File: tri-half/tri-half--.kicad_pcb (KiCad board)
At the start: 2 copper layers, 43.3 x 50 mm, 11 parts, among them J1 Conn_01x05_Pin, J2 Conn_01x05_Pin, J3 Conn_01x05_Pin

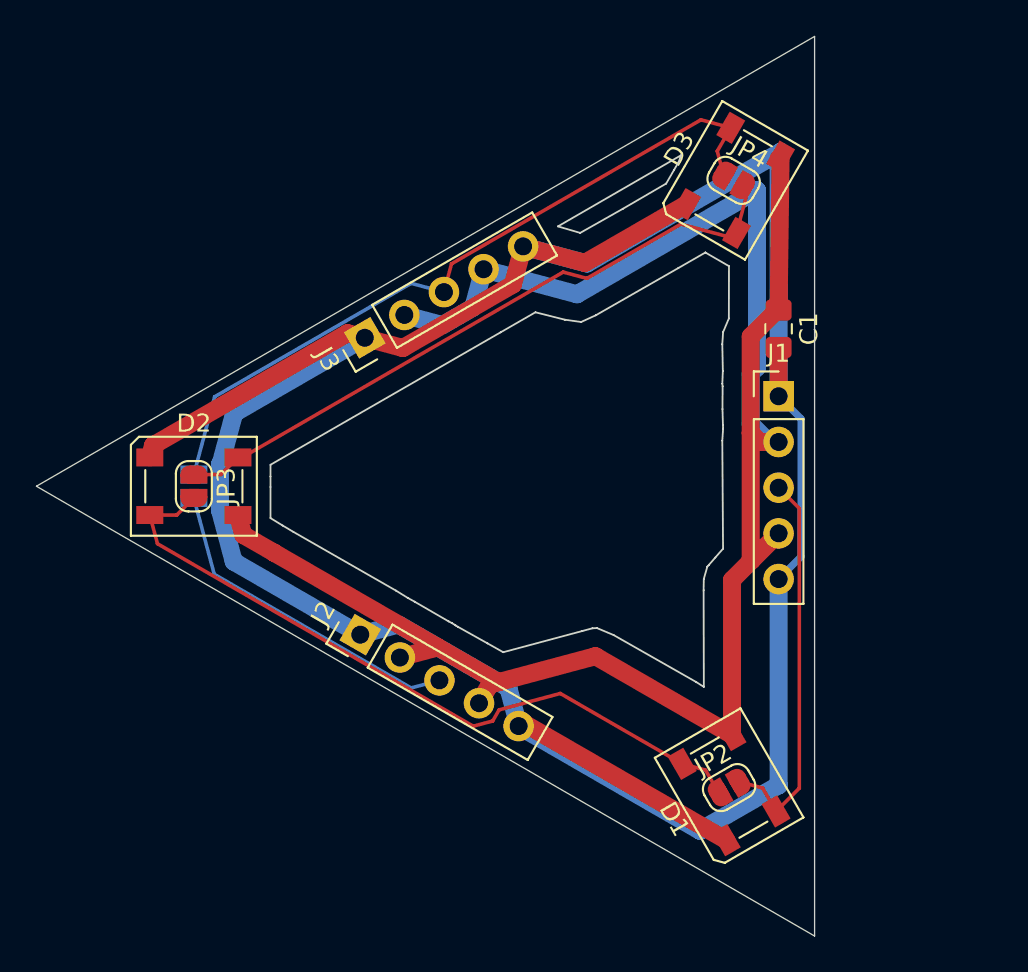
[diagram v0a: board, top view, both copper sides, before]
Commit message: very nice
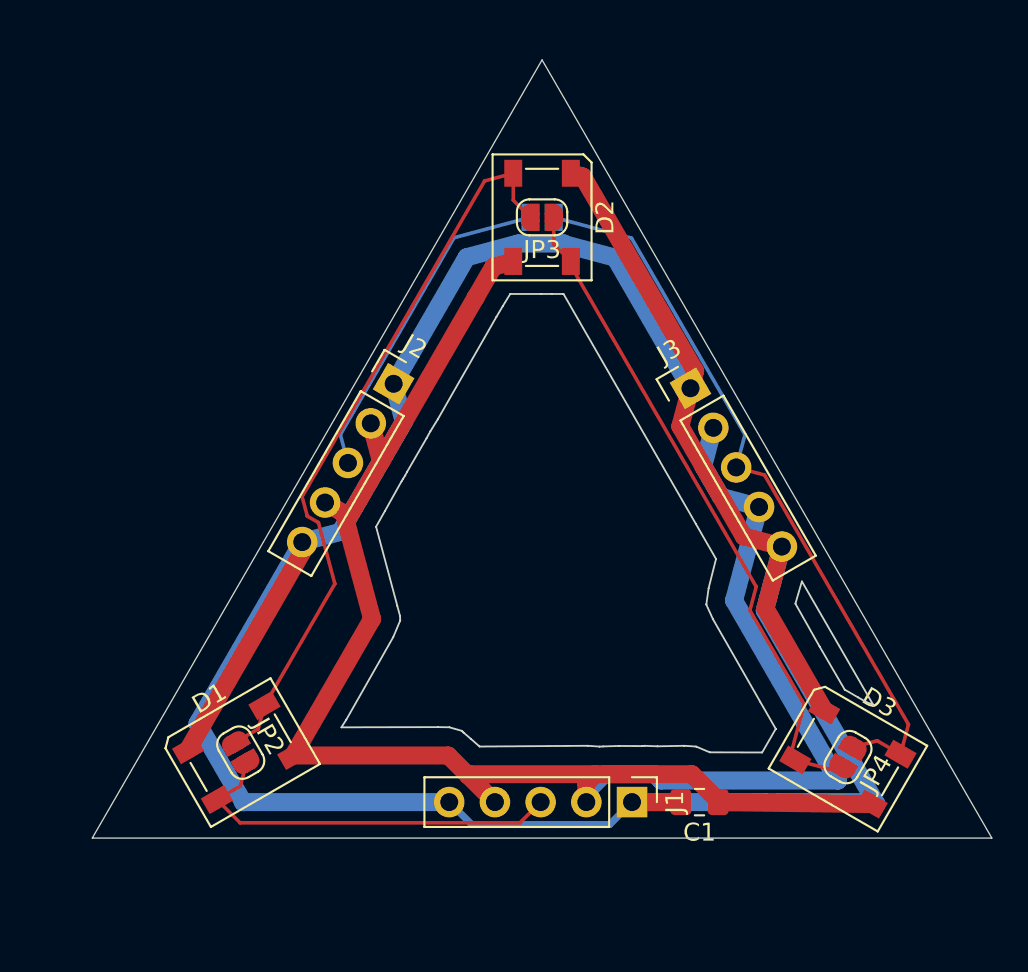
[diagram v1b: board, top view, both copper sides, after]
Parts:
- moved D3 32.7 mm to (116.9, 69.2), turned to -30 degrees
- moved JP4 32.7 mm to (116.9, 69.2), turned to -120 degrees
- moved D1 27.2 mm to (83.1, 68.9), turned to 30 degrees
- moved JP2 27.2 mm to (83.1, 68.9), turned to -60 degrees
- moved C1 26.7 mm to (108.6, 71.7), turned to 180 degrees
- moved JP1 24.5 mm to (99.9, 39.2), turned to 0 degrees
- moved D2 24.5 mm to (99.9, 39.2), turned to -90 degrees
- moved JP3 24.5 mm to (99.9, 39.2), turned to 180 degrees
- moved J1 24.0 mm to (104.9, 71.7), turned to -90 degrees
- moved J3 18.3 mm to (108.1, 48.7), turned to 30 degrees
- moved J2 14.1 mm to (91.6, 48.4), turned to -30 degrees
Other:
- board size 43.3 x 50 mm -> 50 x 43.3 mm
